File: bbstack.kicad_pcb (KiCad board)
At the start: 2 copper layers, 48.1 x 56.4 mm, 6 parts, among them J1 CONN_01X17, J2 CONN_01X16, J3 CONN_01X17, J4 CONN_01X16

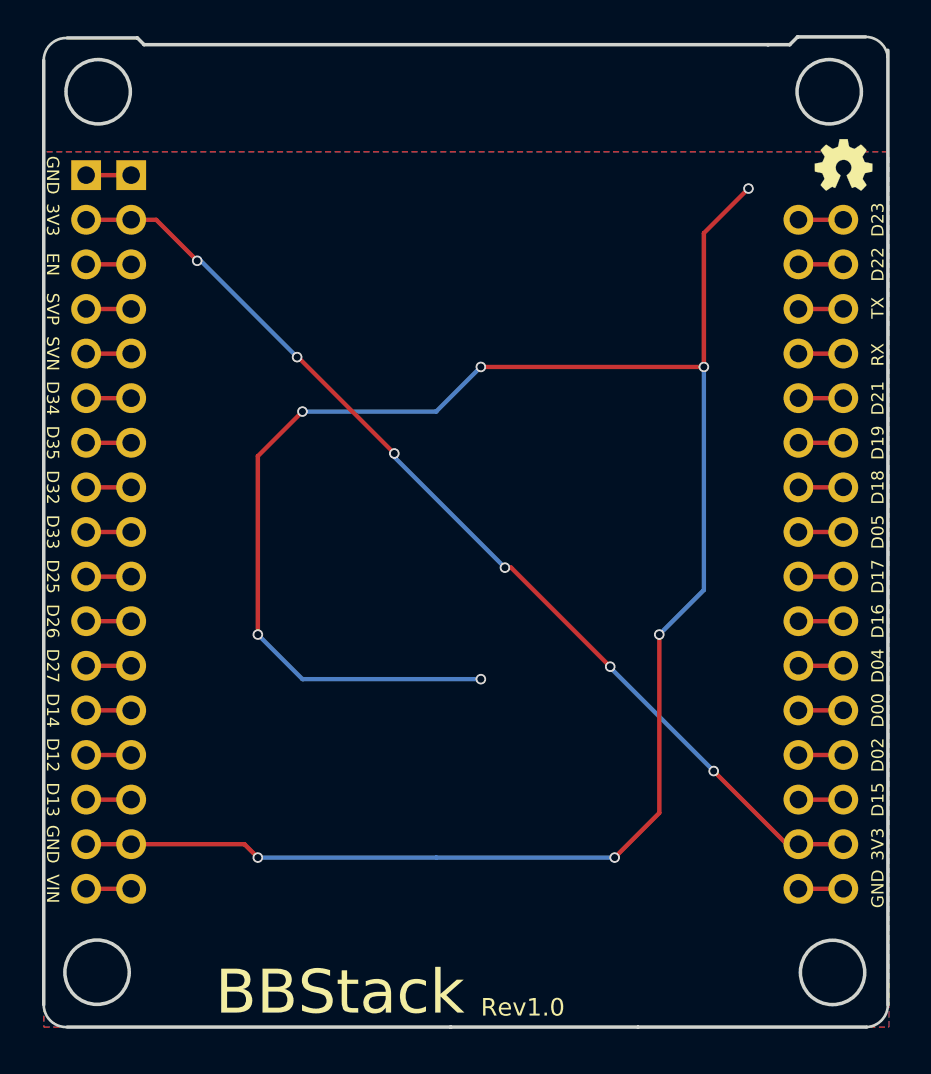
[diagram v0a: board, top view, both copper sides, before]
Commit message: Update to rev1.1
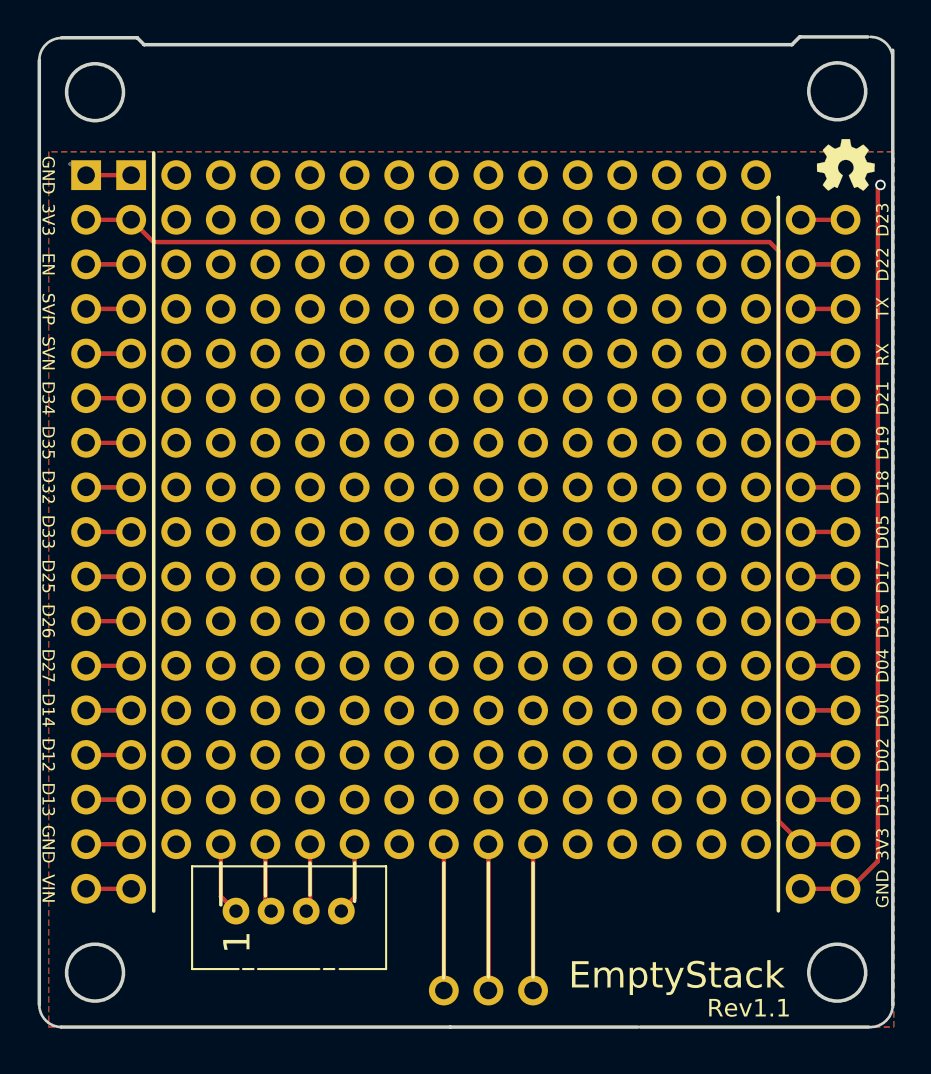
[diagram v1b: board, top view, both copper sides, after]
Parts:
- added J10: CONN_01X14, common:Pin_Header_Straight_1x14_Pitch2.54mm, F.Cu at (155.0, 101.6)
- added J11: CONN_01X14, common:Pin_Header_Straight_1x14_Pitch2.54mm, F.Cu at (155.0, 71.1)
- added J12: CONN_01X14, common:Pin_Header_Straight_1x14_Pitch2.54mm, F.Cu at (155.0, 104.1)
- added J13: CONN_01X14, common:Pin_Header_Straight_1x14_Pitch2.54mm, F.Cu at (155.0, 106.7)
- added J14: CONN_01X14, common:Pin_Header_Straight_1x14_Pitch2.54mm, F.Cu at (155.0, 83.8)
- added J15: CONN_01X14, common:Pin_Header_Straight_1x14_Pitch2.54mm, F.Cu at (155.0, 76.2)
- added J16: CONN_01X14, common:Pin_Header_Straight_1x14_Pitch2.54mm, F.Cu at (155.0, 73.7)
- added J17: CONN_01X14, common:Pin_Header_Straight_1x14_Pitch2.54mm, F.Cu at (155.0, 88.9)
- added J18: CONN_01X14, common:Pin_Header_Straight_1x14_Pitch2.54mm, F.Cu at (155.0, 94.0)
- added J19: CONN_01X14, common:Pin_Header_Straight_1x14_Pitch2.54mm, F.Cu at (155.0, 96.5)
- added J20: CONN_01X14, common:Pin_Header_Straight_1x14_Pitch2.54mm, F.Cu at (155.0, 99.1)
- added J21: CONN_01X03, common:Pin_Header_Straight_1x03_Pitch2.54mm, F.Cu at (175.3, 117.6)
- added J22: grove_01X04, Connectors:Grove_1x04, F.Cu at (158.4, 113.0)
- added J5: CONN_01X14, common:Pin_Header_Straight_1x14_Pitch2.54mm, F.Cu at (155.0, 78.7)
- added J6: CONN_01X14, common:Pin_Header_Straight_1x14_Pitch2.54mm, F.Cu at (155.0, 81.3)
- added J7: CONN_01X14, common:Pin_Header_Straight_1x14_Pitch2.54mm, F.Cu at (155.0, 86.4)
- added J8: CONN_01X14, common:Pin_Header_Straight_1x14_Pitch2.54mm, F.Cu at (155.0, 109.2)
- added J9: CONN_01X14, common:Pin_Header_Straight_1x14_Pitch2.54mm, F.Cu at (155.0, 91.4)
- moved J2 0.13 mm to (193.1, 73.7)
- moved J4 0.13 mm to (190.6, 73.7)
- moved G*** 0.13 mm to (193.1, 70.5) (x2)
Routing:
- net GND: track 129.8 -> 50.3 mm, vias 9 -> 1
- net +3V3: track 58.4 -> 78.1 mm, vias 6 -> 0
- net Net-(J21-Pad3): track 0.00 -> 8.64 mm
- net Net-(J21-Pad2): track 0.00 -> 8.64 mm
- net Net-(J21-Pad1): track 0.00 -> 8.64 mm
- net Net-(J22-Pad1): track 0.00 -> 4.16 mm
- net Net-(J22-Pad4): track 0.00 -> 4.13 mm
- net Net-(J22-Pad2): track 0.00 -> 3.93 mm
- net Net-(J22-Pad3): track 0.00 -> 3.91 mm
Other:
- board size 48.1 x 56.4 mm -> 48.6 x 56.4 mm
- board text added: "EmptyStack"
- board text added: "Rev1.1"
- board text added: "github.com/asukiaaa/emptystack"
- board text removed: "BBStack"
- board text removed: "Rev1.0"
- board text removed: "github.com/asukiaaa/bbstack"
